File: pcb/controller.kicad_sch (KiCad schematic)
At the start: 59 parts, among them J16 uC_NRST, J17 3V3_uC, J18 SWO, J4 DEBUG, J5 UART, U2 SN65HVD234, U3 STM32F103RETx, Y1 8MHz

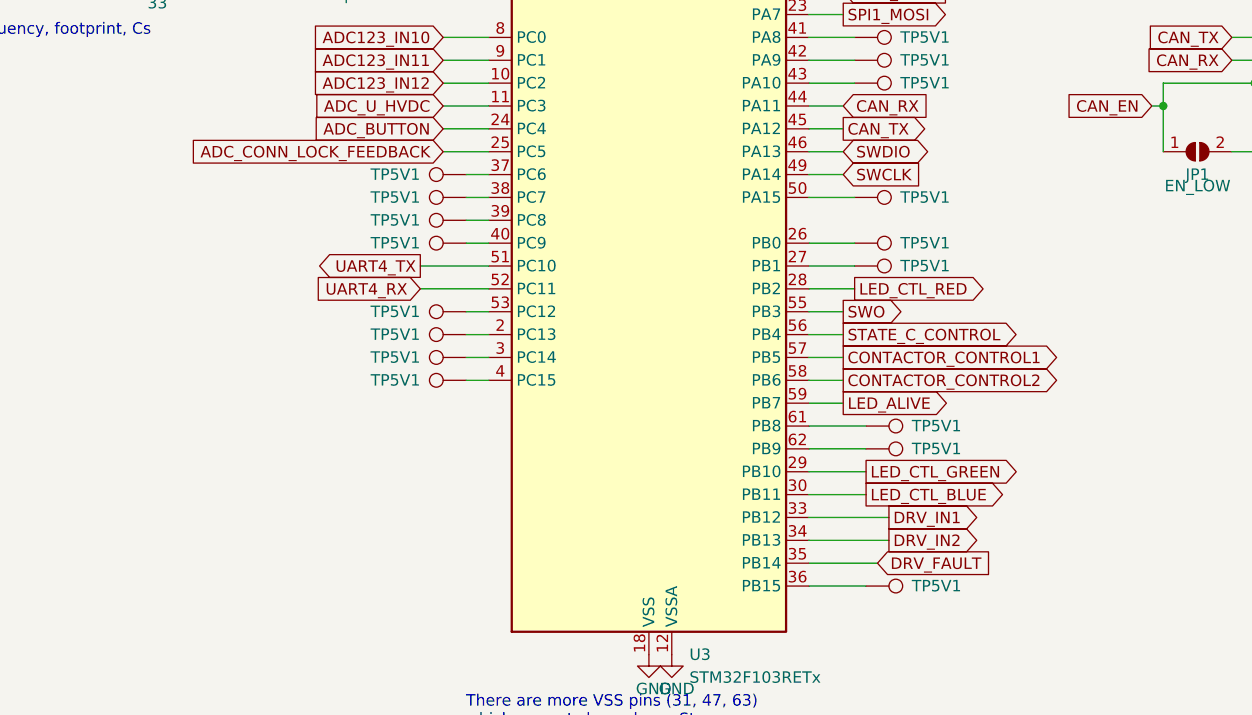
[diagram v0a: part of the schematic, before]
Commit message: routed driver outputs for contactors and lock motor to PWM TIM3 ports. Use protected 12V for DRV.
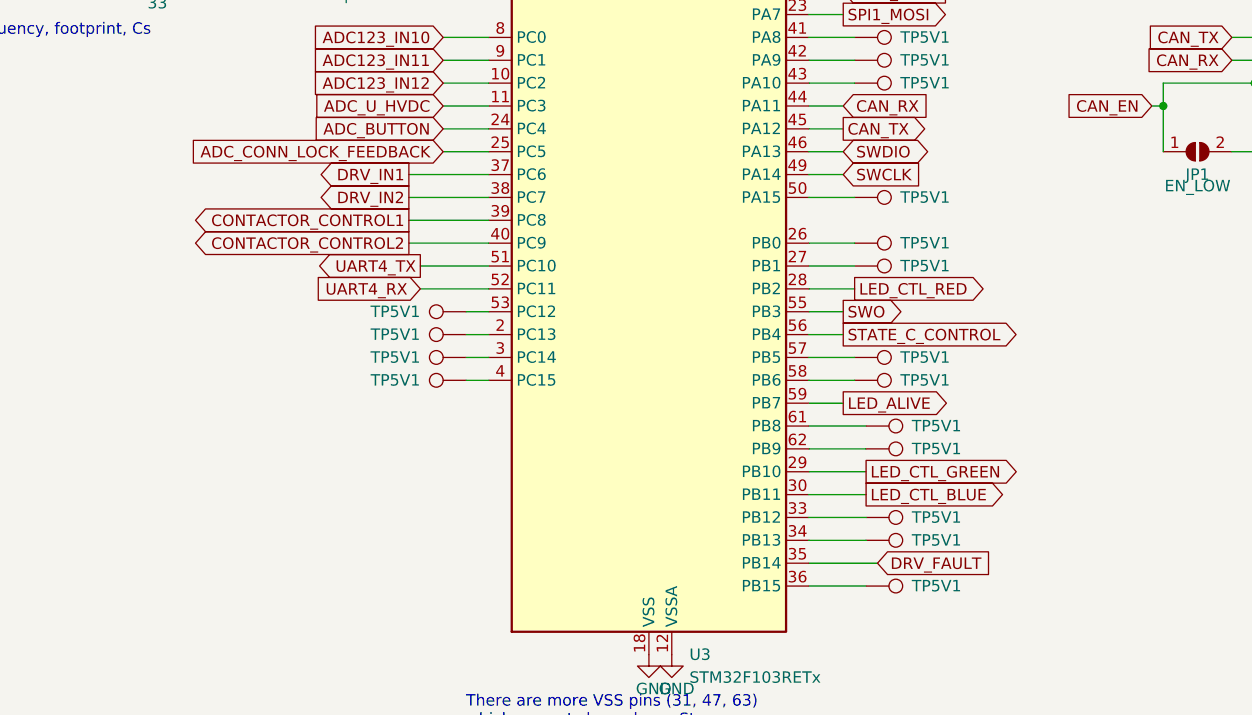
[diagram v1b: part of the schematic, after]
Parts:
- removed TP5V1 (x4): ~, TestPoint:TestPoint_THTPad_D1.0mm_Drill0.5mm, symbol Connector:TestPoint
- added TP5V1 (x4): ~, TestPoint:TestPoint_THTPad_D1.0mm_Drill0.5mm, symbol Connector:TestPoint
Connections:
- net CONTACTOR_CONTROL1: now also U3.39 (PC8); no longer U3.57 (PB5)
- net CONTACTOR_CONTROL2: now also U3.40 (PC9); no longer U3.58 (PB6)
- net DRV_IN1: now also U3.37 (PC6); no longer U3.33 (PB12)
- net DRV_IN2: now also U3.38 (PC7); no longer U3.34 (PB13)
- new net: TP5V1.1, U3.58 (PB6)
- new net: TP5V1.1, U3.33 (PB12)
- new net: TP5V1.1, U3.34 (PB13)
- new net: TP5V1.1, U3.57 (PB5)
